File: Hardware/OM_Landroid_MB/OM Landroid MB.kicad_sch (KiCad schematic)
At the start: 6 parts

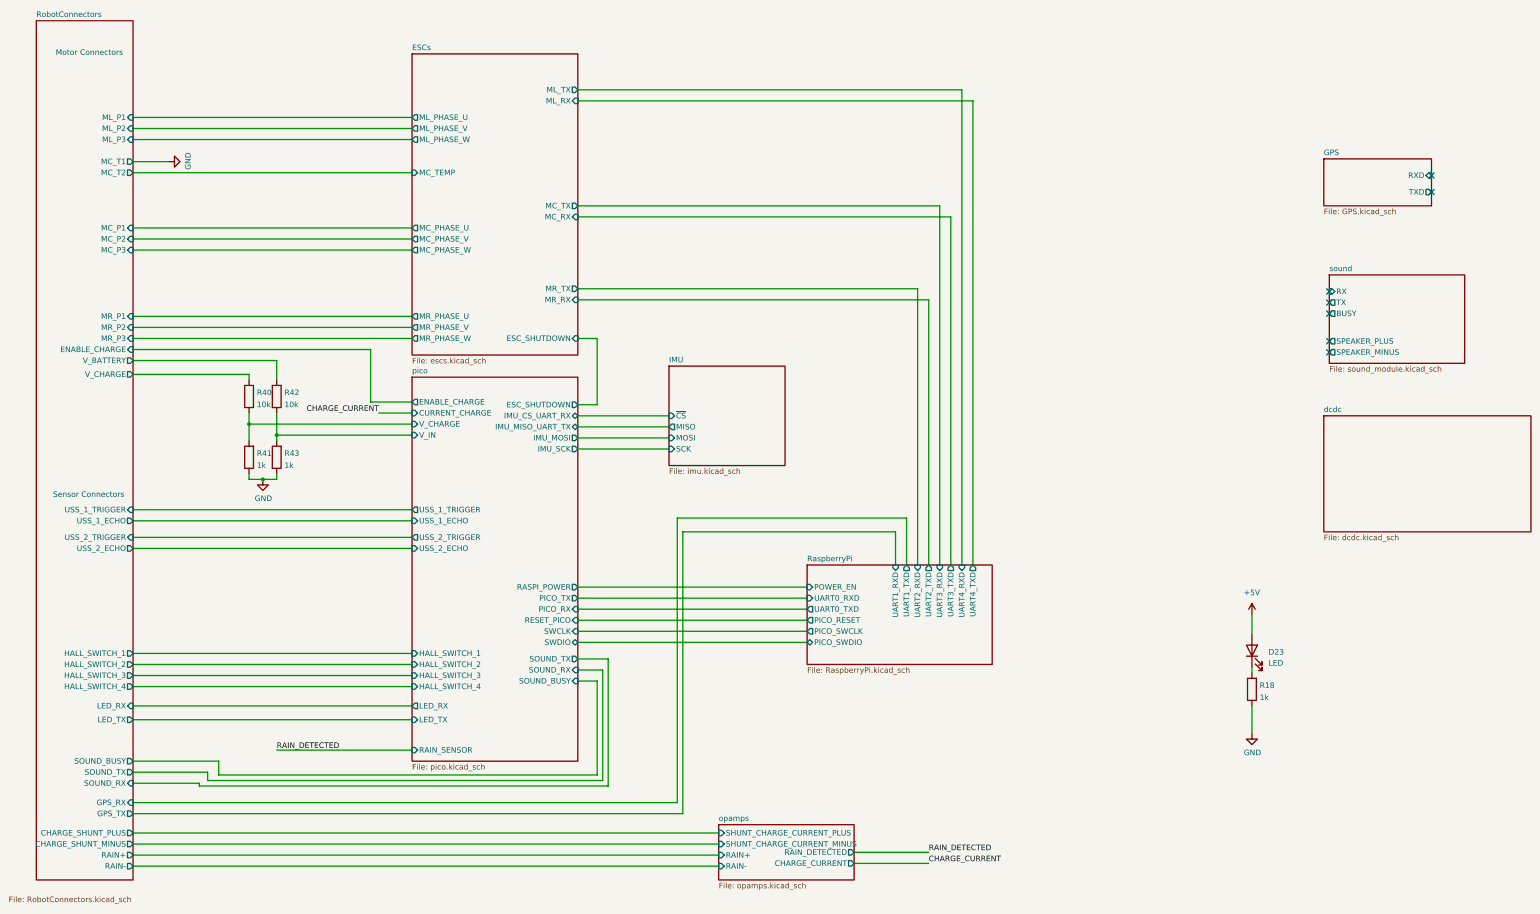
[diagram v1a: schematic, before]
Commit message: Finished Mainboard
Finished Mainboard redesign for OM Landroid
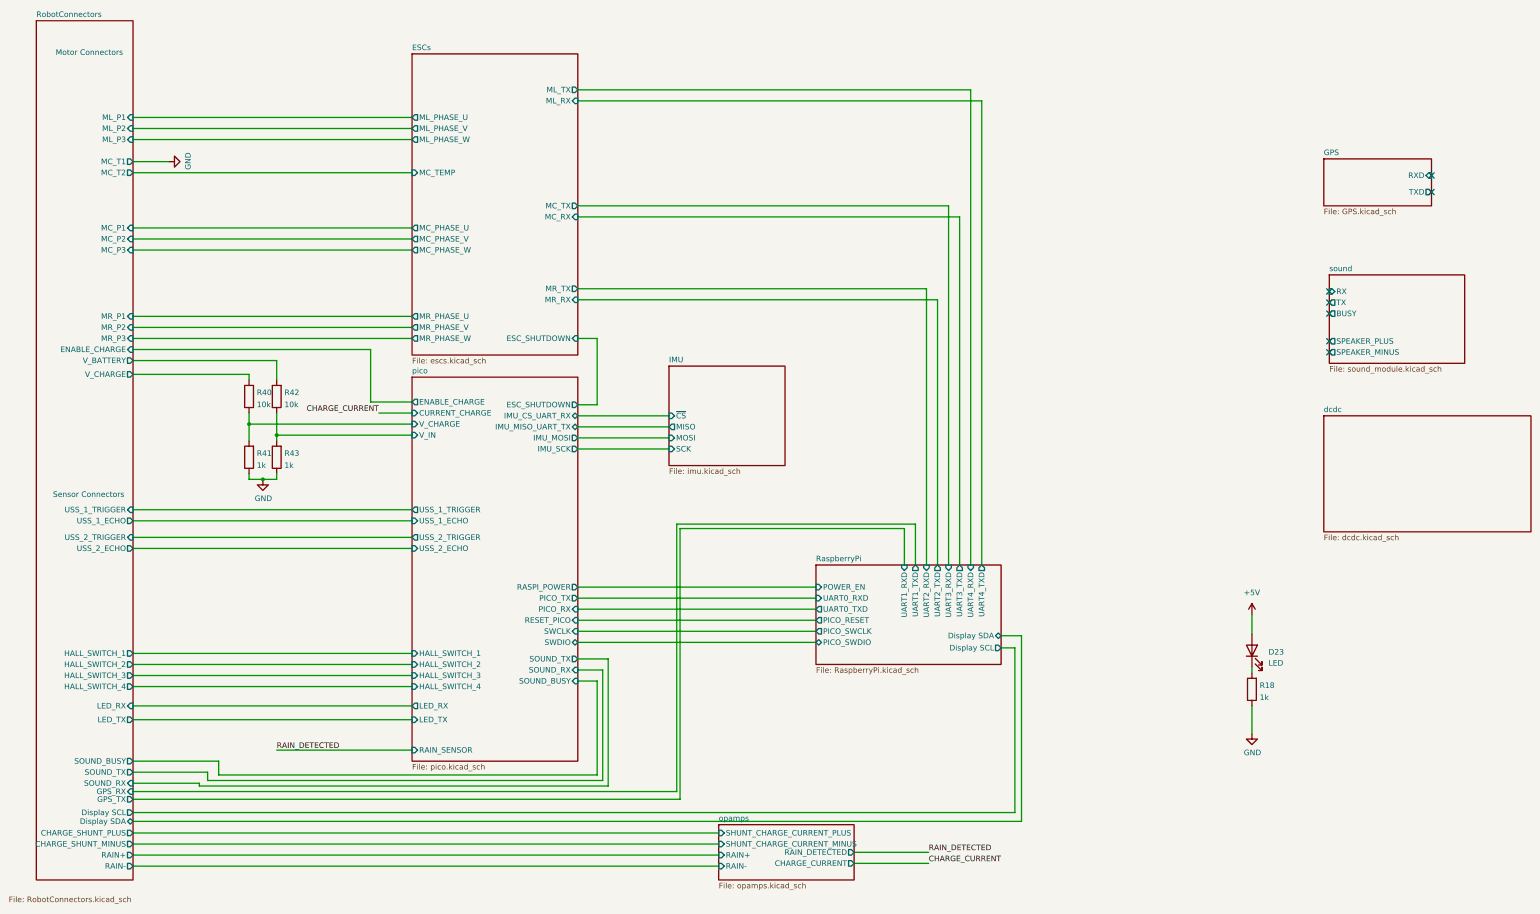
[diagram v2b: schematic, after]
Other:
- sheet RaspberryPi ports: added Display SCL, Display SDA; removed none
- sheet RobotConnectors ports: added Display SCL, Display SDA; removed none
